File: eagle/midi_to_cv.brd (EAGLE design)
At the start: 100.3 x 80 mm, 57 parts, among them IC1 TL074P, IC2 4504N, IC3 4099N, IC4 TL074P, U1 ATMEGA328P_PDIP

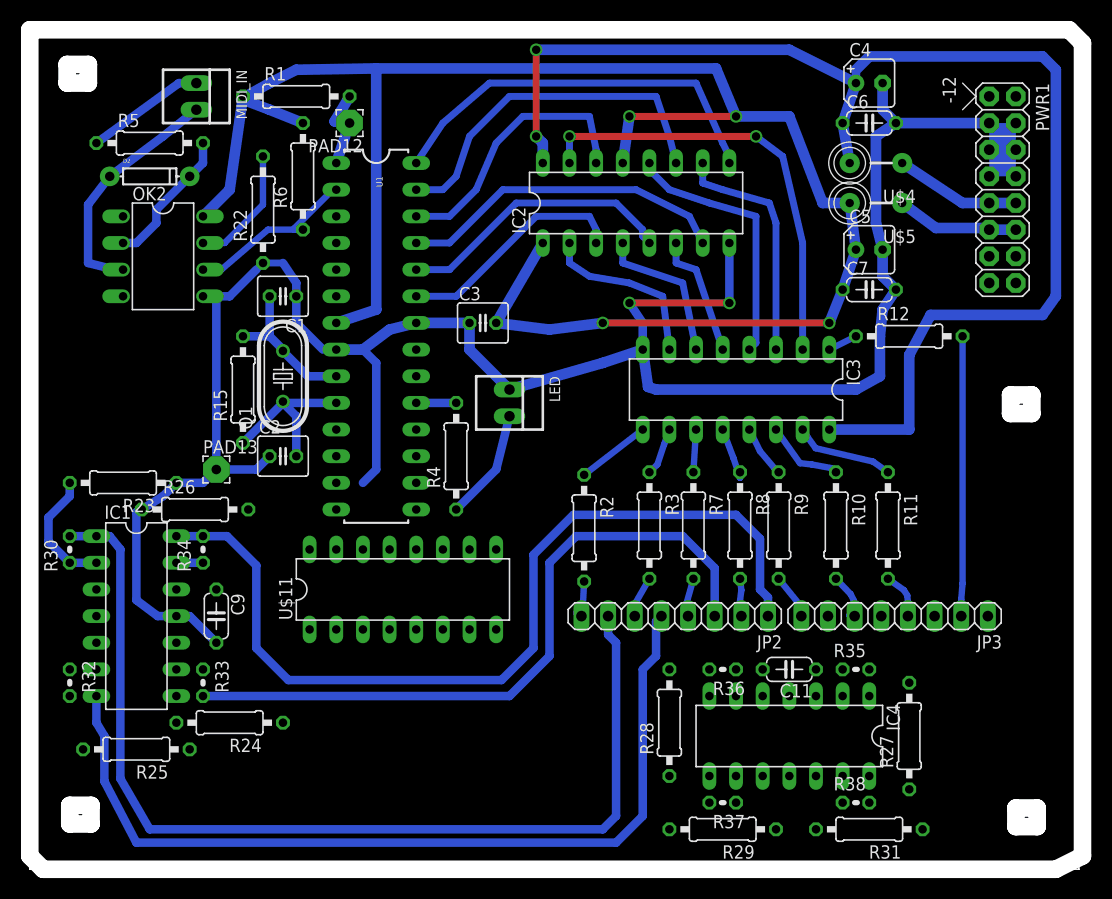
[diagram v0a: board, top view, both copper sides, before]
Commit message: reverted to working midi board
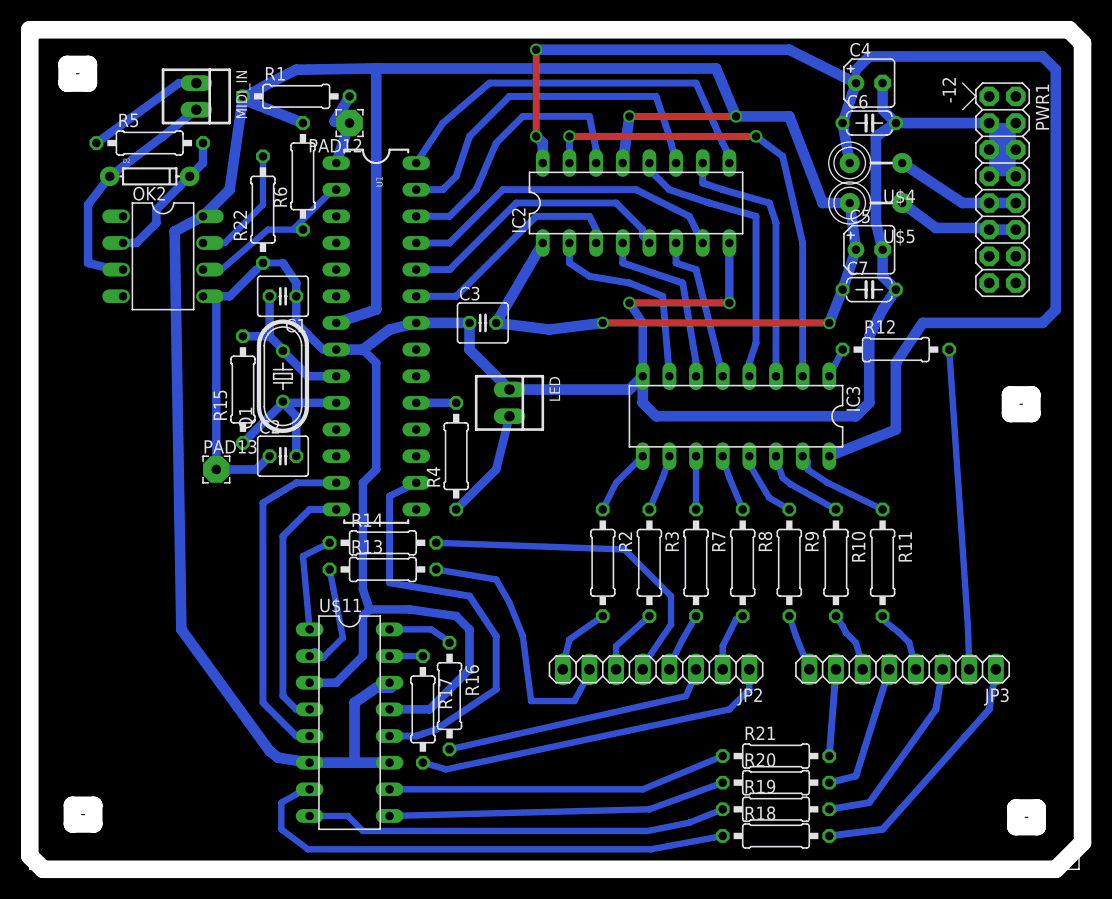
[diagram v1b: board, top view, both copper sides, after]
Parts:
- removed C11, C9: 100n, rcl:C050-024X044
- removed IC1, IC4: TL074P, linear:DIL14
- removed R23, R24, R25, R26, R27, R28, R29, R31: 1k, rcl:0207/10
- removed R30, R32, R33, R34, R35, R36, R37, R38: 1k8, rcl:0204V
- added R13, R14, R16, R17, R18, R19, R20, R21: 1k, rcl:0207/10
- R22: value 1k -> 2k4
- R6: value 470 -> 270
- moved U$11 13.7 mm to (30.5, 14.0), turned to 270 degrees
- moved JP2 5.38 mm to (59.7, 19.1)
- moved JP3 5.14 mm to (83.2, 19.1)
- moved R2 3.75 mm to (54.6, 29.2)
- moved R9 3.70 mm to (72.4, 29.2)
- moved R11 3.59 mm to (81.3, 29.2)
- moved R7 3.57 mm to (63.5, 29.2)
- moved R8 3.57 mm to (67.9, 29.2)
- moved R10 3.56 mm to (76.8, 29.2)
- moved R3 3.56 mm to (59.1, 29.2)
- moved IC3 2.54 mm to (67.3, 43.2)
- moved R12 1.80 mm to (82.5, 49.5)
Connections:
- removed net N$43: IC4.12, U$11.10
- removed net N$63: IC1.13, R26.2, R34.1
- removed net N$64: IC4.2, R27.2, R35.1
- removed net N$65: IC4.6, R28.2, R36.1
- removed net N$66: IC4.9, R29.2, R37.1
- removed net N$67: IC4.13, R31.2, R38.1
- removed net N$68: IC1.12, U$11.15
- removed net N$69: IC1.10, U$11.16
- removed net N$70: IC1.5, U$11.1
- removed net N$71: IC1.3, U$11.2
- new net N$24: JP2.5, R14.2
- new net N$40: JP3.1, R18.2
- net +12V: no longer C11.1, C9.1, IC1.4, IC4.4
- net GND: no longer C11.2, C9.2, IC1.11, IC4.11, R23.1, R24.1, R25.1, R26.1, R27.1, R28.1, R29.1, R31.1
- net N$22: now also R13.2; no longer IC1.1, R30.2
- net N$28: now also R16.2; no longer IC1.8, R33.2
- net N$29: now also R17.2; no longer IC1.14, R34.2
- net N$34: now also R20.2; no longer IC4.8, R37.2
- net N$41: now also R19.2; no longer IC4.7, R36.2
- net N$51: now also R21.2; no longer IC4.14, R38.2
- net N$52: now also R13.1, U$11.2; no longer IC4.1, JP3.1, R35.2
- net N$53: now also R14.1, U$11.1; no longer IC4.10, U$11.9
- net N$54: now also R16.1, U$11.16; no longer IC4.5, U$11.8
- net N$55: now also R17.1, U$11.15; no longer IC4.3, U$11.7
- net N$56: now also R18.1, U$11.7; no longer IC1.7, JP2.5, R32.2
- net N$57: now also R19.1, U$11.8; no longer IC1.2, R23.2, R30.1
- net N$58: now also R20.1, U$11.9; no longer IC1.9, R24.2, R33.1
- net N$59: now also R21.1, U$11.10; no longer IC1.6, R25.2, R32.1
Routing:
- net +5V: track 180.8 -> 258.0 mm
- net N$22: track 97.2 -> 25.5 mm
- net N$29: track 86.3 -> 34.5 mm
- net N$28: track 66.1 -> 25.8 mm
- net N$15: track 0.00 -> 39.9 mm
- net N$56: track 84.0 -> 48.5 mm
- net N$59: track 0.00 -> 32.4 mm
- net N$14: track 0.00 -> 32.3 mm
- net N$58: track 0.00 -> 32.2 mm
- net N$24: track 0.00 -> 32.1 mm
- net N$57: track 11.8 -> 40.3 mm
- net N$27: track 0.00 -> 24.4 mm
- net N$40: track 0.00 -> 24.3 mm
- net GND: track 202.5 -> 226.4 mm
- net N$41: track 0.00 -> 18.7 mm
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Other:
- outline, holes or cut-outs redrawn
